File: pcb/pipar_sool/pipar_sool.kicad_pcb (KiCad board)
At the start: 2 copper layers, 139.4 x 109.8 mm, 109 parts, among them M2 MountingHole_2.2mm_M2, SW1 SW_Wuerth_450301014042

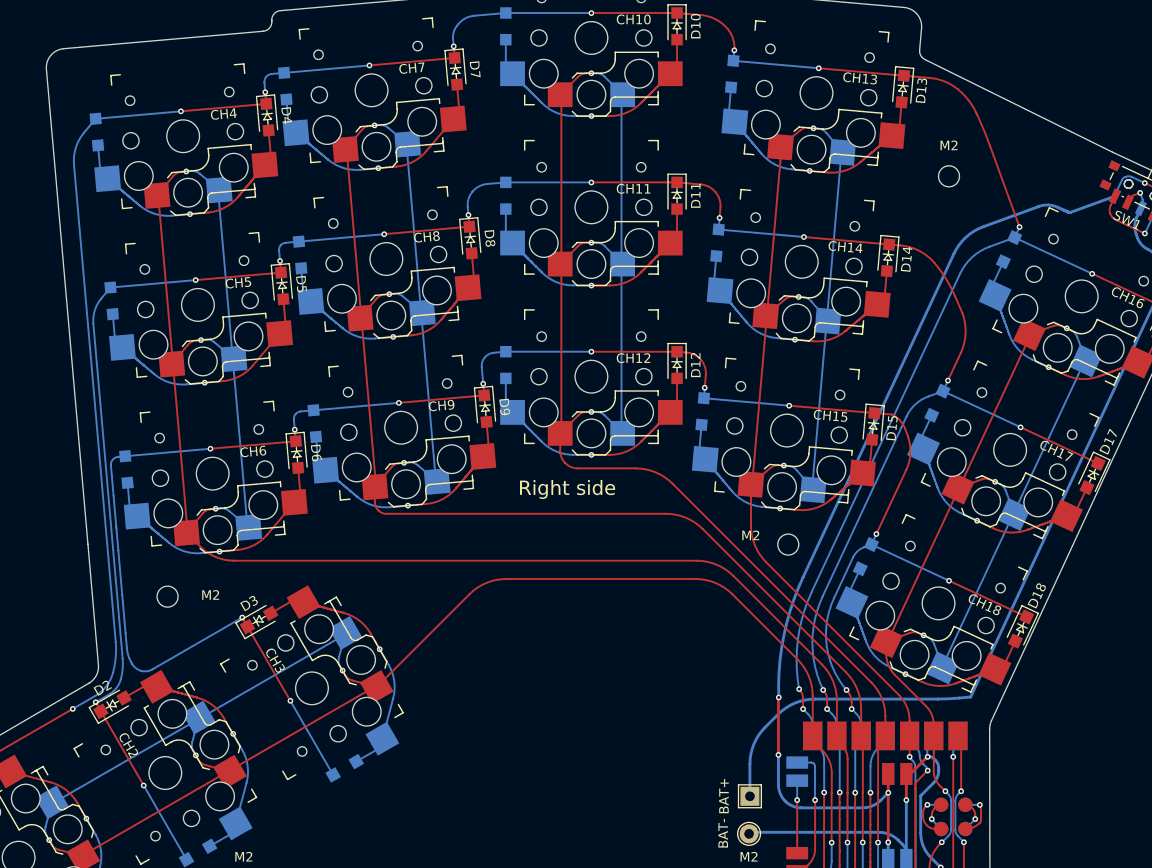
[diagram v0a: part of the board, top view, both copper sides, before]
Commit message: starts work on t460s board 2
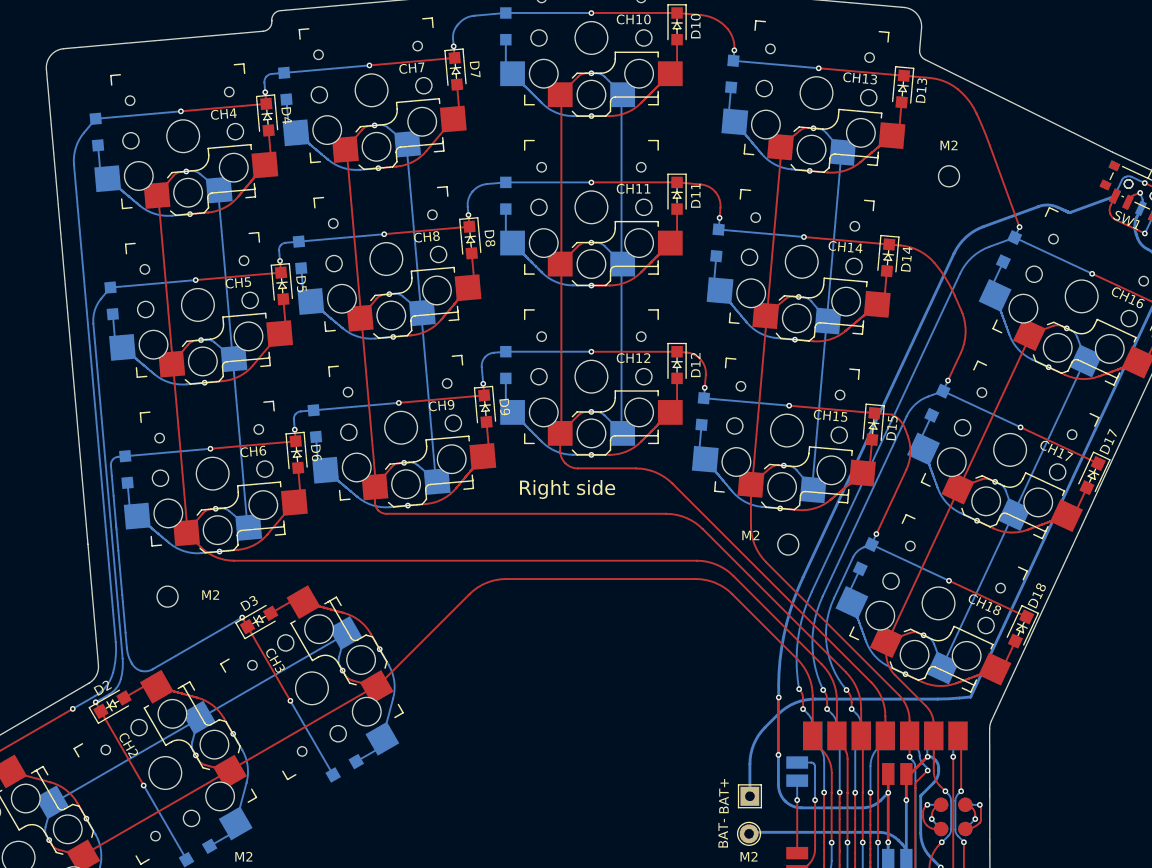
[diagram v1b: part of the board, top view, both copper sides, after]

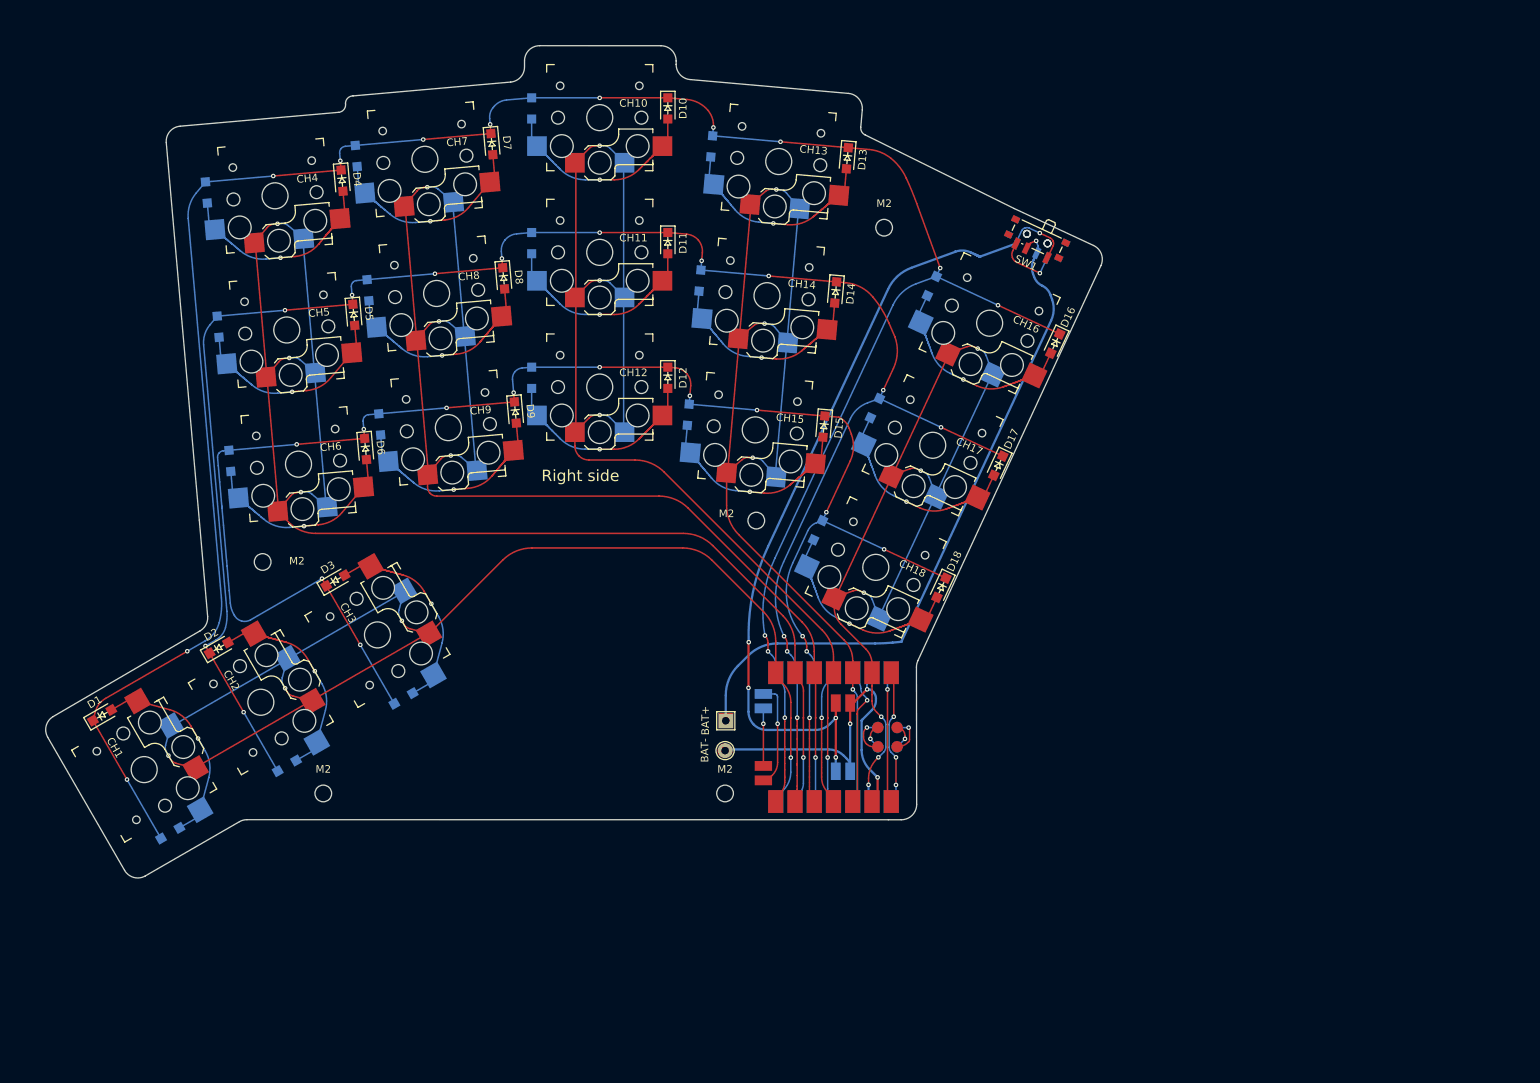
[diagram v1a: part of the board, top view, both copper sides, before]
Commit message: Recreated Sool & Pipar for production run
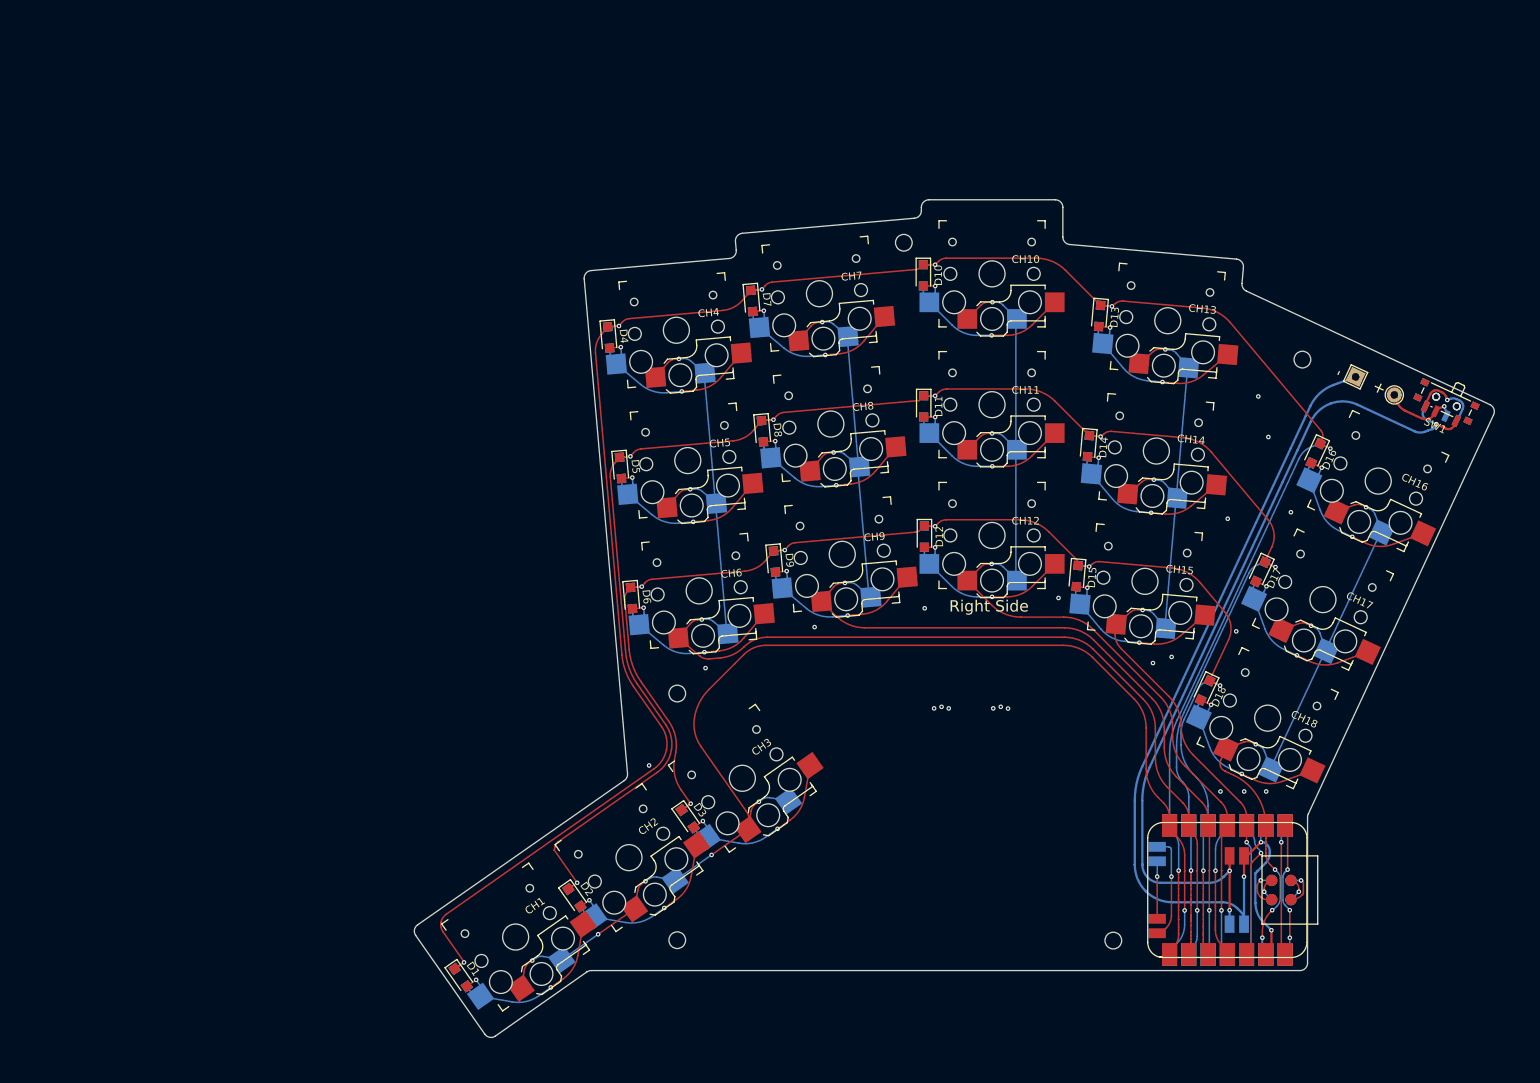
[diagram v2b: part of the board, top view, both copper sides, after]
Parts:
- removed ? (x44): , 
- removed the D1 at (20.3, 105.5)
- removed the D1 at (29.3, 121.1)
- removed the D10 at (94.9, 25.5)
- removed the D10 at (76.9, 25.5)
- removed the D11 at (94.9, 43.2)
- removed the D11 at (76.9, 43.2)
- removed the D12 at (94.9, 61.0)
- removed the D12 at (76.9, 61.0)
- removed the D13 at (118.6, 32.0)
- removed the D13 at (100.7, 30.5)
- removed the D14 at (117.0, 49.7)
- removed the D14 at (99.1, 48.2)
- removed the D15 at (115.5, 67.4)
- removed the D15 at (97.6, 65.9)
- removed the D16 at (146.0, 56.5)
- removed the D16 at (129.7, 48.9)
- removed the D17 at (138.5, 72.6)
- removed the D17 at (122.2, 65.0)
- removed the D18 at (131.0, 88.7)
- removed the D18 at (114.7, 81.1)
- removed the D2 at (35.7, 96.6)
- removed the D2 at (44.6, 112.2)
- removed the D3 at (51.0, 87.7)
- removed the D3 at (60.0, 103.3)
- removed the D4 at (51.9, 35.0)
- removed the D4 at (34.0, 36.6)
- removed the D5 at (53.5, 52.7)
- removed the D5 at (35.6, 54.3)
- removed the D6 at (55.0, 70.4)
- removed the D6 at (37.1, 72.0)
- removed the D7 at (71.7, 30.2)
- removed the D7 at (53.8, 31.7)
- removed the D8 at (73.2, 47.9)
- removed the D8 at (55.3, 49.4)
- removed the D9 at (74.8, 65.6)
- removed the D9 at (56.9, 67.1)
- removed M2 (x5): MountingHole_2.2mm_M2, MountingHole:MountingHole_2.2mm_M2
- removed REF** (x2): Salt & Pepper, Art:Salt
- removed the SW1 at (143.5, 42.9) (x2)
- added D1: D, Diode_SMD:Nexperia_CFP3_SOD-123W, F.Cu at (67.6, 140.1)
- added D1: D, Diode_SMD:Nexperia_CFP3_SOD-123W, B.Cu at (67.6, 140.1)
- added D10: D, Diode_SMD:Nexperia_CFP3_SOD-123W, F.Cu at (128.6, 47.5)
- added D10: D, Diode_SMD:Nexperia_CFP3_SOD-123W, B.Cu at (128.6, 47.5)
- added D11: D, Diode_SMD:Nexperia_CFP3_SOD-123W, F.Cu at (128.6, 64.8)
- added D11: D, Diode_SMD:Nexperia_CFP3_SOD-123W, B.Cu at (128.6, 64.8)
- added D12: D, Diode_SMD:Nexperia_CFP3_SOD-123W, F.Cu at (128.7, 81.9)
- added D12: D, Diode_SMD:Nexperia_CFP3_SOD-123W, B.Cu at (128.7, 81.9)
- added D13: D, Diode_SMD:Nexperia_CFP3_SOD-123W, F.Cu at (151.8, 52.8)
- added D13: D, Diode_SMD:Nexperia_CFP3_SOD-123W, B.Cu at (151.8, 52.8)
- added D14: D, Diode_SMD:Nexperia_CFP3_SOD-123W, F.Cu at (150.4, 70.0)
- added D14: D, Diode_SMD:Nexperia_CFP3_SOD-123W, B.Cu at (150.4, 70.0)
- added D15: D, Diode_SMD:Nexperia_CFP3_SOD-123W, F.Cu at (148.9, 87.2)
- added D15: D, Diode_SMD:Nexperia_CFP3_SOD-123W, B.Cu at (148.9, 87.2)
- added D16: D, Diode_SMD:Nexperia_CFP3_SOD-123W, F.Cu at (180.3, 70.9)
- added D16: D, Diode_SMD:Nexperia_CFP3_SOD-123W, B.Cu at (180.3, 70.9)
- added D17: D, Diode_SMD:Nexperia_CFP3_SOD-123W, F.Cu at (173.1, 86.6)
- added D17: D, Diode_SMD:Nexperia_CFP3_SOD-123W, B.Cu at (173.1, 86.6)
- added D18: D, Diode_SMD:Nexperia_CFP3_SOD-123W, F.Cu at (165.8, 102.2)
- added D18: D, Diode_SMD:Nexperia_CFP3_SOD-123W, B.Cu at (165.8, 102.2)
- added D2: D, Diode_SMD:Nexperia_CFP3_SOD-123W, F.Cu at (82.6, 129.6)
- added D2: D, Diode_SMD:Nexperia_CFP3_SOD-123W, B.Cu at (82.6, 129.6)
- added D3: D, Diode_SMD:Nexperia_CFP3_SOD-123W, F.Cu at (97.5, 119.2)
- added D3: D, Diode_SMD:Nexperia_CFP3_SOD-123W, B.Cu at (97.5, 119.2)
- added D4: D, Diode_SMD:Nexperia_CFP3_SOD-123W, F.Cu at (87.1, 55.7)
- added D4: D, Diode_SMD:Nexperia_CFP3_SOD-123W, B.Cu at (87.1, 55.7)
- added D5: D, Diode_SMD:Nexperia_CFP3_SOD-123W, F.Cu at (88.6, 72.9)
- added D5: D, Diode_SMD:Nexperia_CFP3_SOD-123W, B.Cu at (88.6, 72.9)
- added D6: D, Diode_SMD:Nexperia_CFP3_SOD-123W, F.Cu at (90.1, 90.1)
- added D6: D, Diode_SMD:Nexperia_CFP3_SOD-123W, B.Cu at (90.1, 90.1)
- added D7: D, Diode_SMD:Nexperia_CFP3_SOD-123W, F.Cu at (106.0, 50.9)
- added D7: D, Diode_SMD:Nexperia_CFP3_SOD-123W, B.Cu at (106.0, 50.9)
- added D8: D, Diode_SMD:Nexperia_CFP3_SOD-123W, F.Cu at (107.4, 68.1)
- added D8: D, Diode_SMD:Nexperia_CFP3_SOD-123W, B.Cu at (107.4, 68.1)
- added D9: D, Diode_SMD:Nexperia_CFP3_SOD-123W, F.Cu at (109.0, 85.2)
- added D9: D, Diode_SMD:Nexperia_CFP3_SOD-123W, B.Cu at (109.0, 85.2)
- added SW1: SW_Wuerth_450301014042, Button_Switch_SMD:SW_SPDT_PCM12, F.Cu at (197.5, 64.4)
- added SW1: SW_Wuerth_450301014042, Button_Switch_SMD:SW_SPDT_PCM12, B.Cu at (197.5, 64.4)
- added U1: Seeeduino Xiao nRF52840, Seeed Studio XIAO Series Library:XIAO-nRF52840-Sense-14P-2.54-21X17.8MM, F.Cu at (168.7, 128.6)
- added U1: Seeeduino Xiao nRF52840, Seeed Studio XIAO Series Library:XIAO-nRF52840-Sense-14P-2.54-21X17.8MM, B.Cu at (168.7, 128.6)
- added U2: ~, MountingHole:MountingHole_2.2mm_M2, F.Cu at (96.1, 102.6)
- added U3: ~, MountingHole:MountingHole_2.2mm_M2, F.Cu at (126.0, 43.2)
- added U4: ~, MountingHole:MountingHole_2.2mm_M2, F.Cu at (178.6, 58.6)
- added U5: ~, MountingHole:MountingHole_2.2mm_M2, F.Cu at (96.1, 135.2)
- added U6: ~, MountingHole:MountingHole_2.2mm_M2, F.Cu at (153.6, 135.2)
- added U7: ~, Art:Salt, F.Cu at (134.9, 117.9)
- added U7: ~, Art:Salt, B.Cu at (134.9, 117.9)
- TP1: footprint TestPoint:TestPoint_THTPad_D2.0mm_Drill1.0mm -> TestPoint:TestPoint_THTPad_2.0x2.0mm_Drill1.0mm
- TP2: footprint TestPoint:TestPoint_THTPad_2.0x2.0mm_Drill1.0mm -> TestPoint:TestPoint_THTPad_D2.0mm_Drill1.0mm
- moved TP2 98.1 mm to (190.7, 63.3), turned to 65 degrees
- moved TP1 96.7 mm to (185.6, 60.9), turned to 65 degrees
- moved CH4 55.8 mm to (96.0, 54.7)
- moved CH10 55.7 mm to (137.7, 47.3)
- moved CH5 55.6 mm to (97.5, 71.9)
- moved CH11 55.5 mm to (137.7, 64.5)
- moved CH13 55.4 mm to (160.8, 53.5)
- moved CH6 55.4 mm to (99.0, 89.1)
- moved CH18 55.4 mm to (174.0, 105.9)
- moved CH17 55.3 mm to (181.3, 90.3)
- moved CH12 55.3 mm to (137.7, 81.8)
- moved CH16 55.3 mm to (188.6, 74.6)
- moved CH14 55.3 mm to (159.3, 70.7)
- moved CH15 55.1 mm to (157.8, 87.8)
- moved CH7 55.0 mm to (114.9, 49.9)
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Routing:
- net Net-(SW1-C): track 90.4 -> 10.1 mm
- net GND: track 50.0 -> 123.5 mm, vias 3 -> 24
- net Net-(D12-K): track 220.8 -> 178.6 mm, vias 14 -> 7
- net Net-(U1-P0.28): track 146.3 -> 109.7 mm
- net Net-(U1-P0.29): track 163.9 -> 128.4 mm
- net Net-(U1-P0.03): track 129.3 -> 95.0 mm
- net Net-(U1-P0.04): track 178.8 -> 144.5 mm
- net Net-(U1-P0.05): track 193.3 -> 162.4 mm
- net Net-(D11-K): track 253.2 -> 236.5 mm, vias 14 -> 7
- net Net-(D1-K): track 312.1 -> 296.6 mm, vias 14 -> 7
- net Net-(U1-P1.11): track 174.3 -> 166.8 mm, vias 4 -> 6
- net Net-(SW1-B): track 110.0 -> 111.3 mm, vias 5 -> 3
- net unconnected-(SW1-A-Pad3): track 8.43 -> 9.67 mm
- net Net-(D2-A): track 27.5 -> 26.9 mm, vias 1 -> 2
- net Net-(D5-A): track 27.4 -> 26.9 mm, vias 1 -> 2
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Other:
- board size 139.4 x 109.8 mm -> 142.4 x 110.5 mm
- board text added: "+"
- board text added: "-"
- board text added: "Left Side"
- board text added: "Right Side"
- board text removed: "BAT+"
- board text removed: "BAT-"
- board text removed: "Right side"
